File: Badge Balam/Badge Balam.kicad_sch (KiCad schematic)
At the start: 4 parts, among them SW2 SW_SPDT

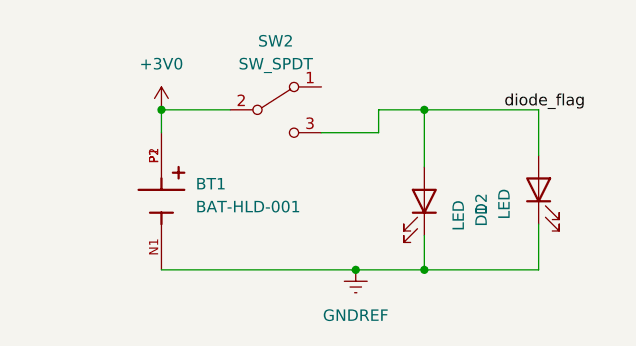
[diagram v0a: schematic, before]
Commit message: cambios
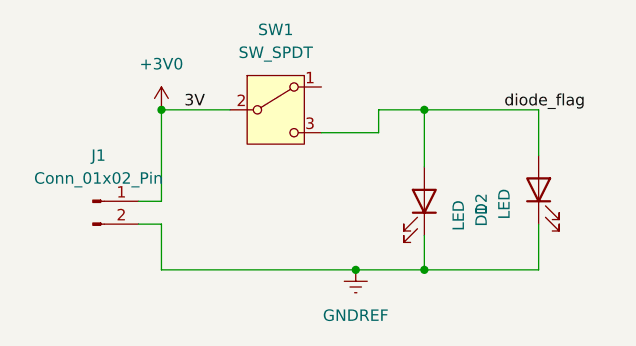
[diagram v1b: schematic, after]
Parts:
- removed BT1: BAT-HLD-001, Battery:BatteryHolder_Keystone_3002_1x2032, symbol Battery Holder:BAT-HLD-001
- removed SW2: SW_SPDT, symbol Switch:SW_SPDT
- added J1: Conn_01x02_Pin, TerminalBlock_MetzConnect:TerminalBlock_MetzConnect_Type073_RT02602HBLU_1x02_P5.08mm_Horizontal, symbol Connector:Conn_01x02_Pin
- added SW1: SW_SPDT, Button_Switch_THT:SW_E-Switch_EG1271_SPDT, symbol Switch:SW_SPDT
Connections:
- net +3V0: now also J1.1 (Pin_1), SW1.2 (B)
- net GNDREF: now also J1.2 (Pin_2)
- net diode_flag: now also SW1.3 (C)
